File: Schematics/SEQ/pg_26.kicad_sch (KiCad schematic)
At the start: 4 parts, among them U2701 F374, U2702 F374, U2703 F374, U2704 F20

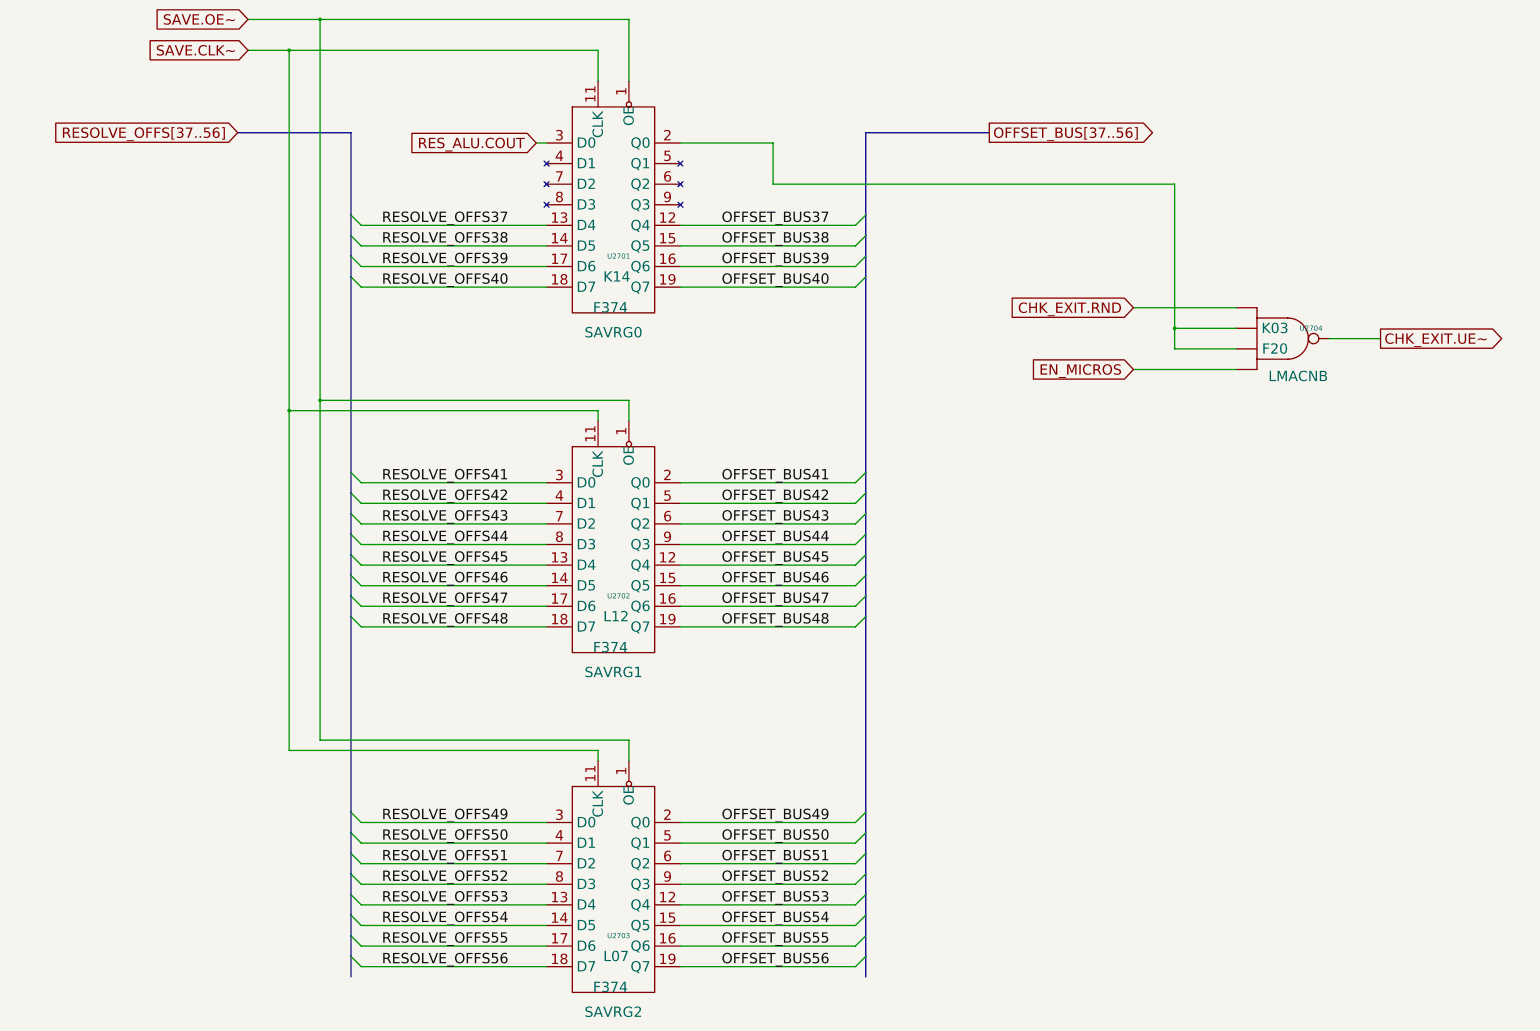
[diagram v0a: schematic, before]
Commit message: Much work on SEQ
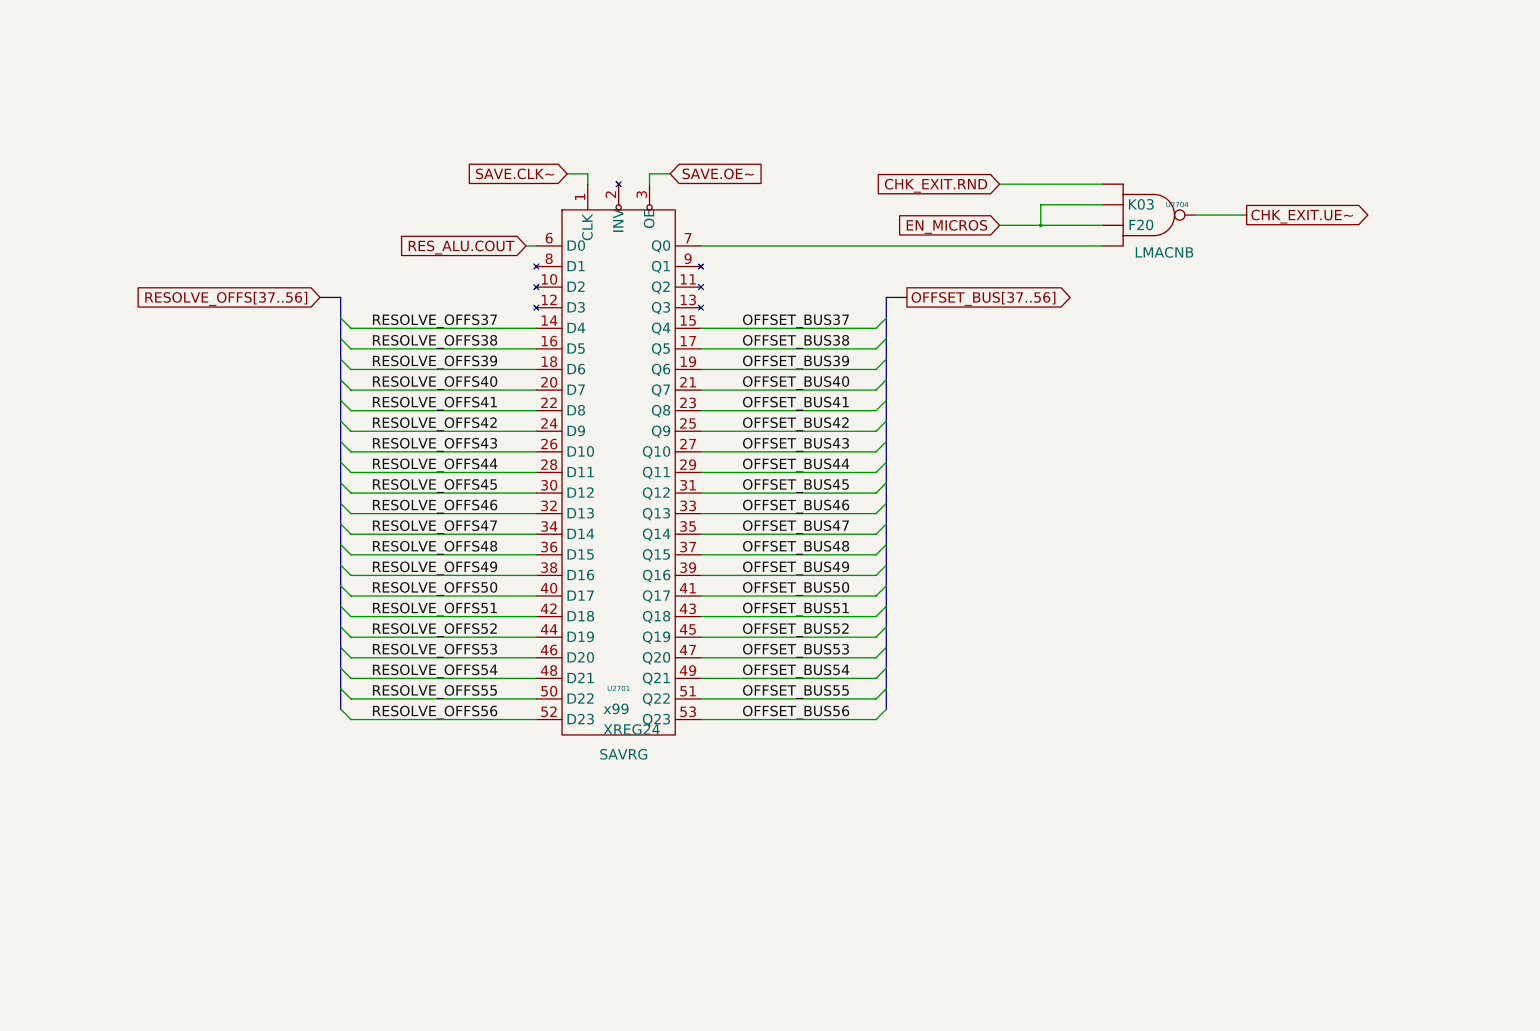
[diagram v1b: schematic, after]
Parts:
- removed U2702, U2703: F374, symbol r1000:F374
- U2701: value F374 -> XREG24; symbol r1000:F374 -> r1000:XREG24; Location K14 -> x99; Name SAVRG0 -> SAVRG
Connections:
- net EN_MICROS: now also U2704.2 (D1), U2704.4 (D2); no longer U2704.5 (D3)
- net OFFSET_BUS37: now also U2701.15 (Q4); no longer U2701.12 (Q4)
- net OFFSET_BUS38: now also U2701.17 (Q5); no longer U2701.15 (Q5)
- net OFFSET_BUS39: now also U2701.19 (Q6); no longer U2701.16 (Q6)
- net OFFSET_BUS40: now also U2701.21 (Q7); no longer U2701.19 (Q7)
- net OFFSET_BUS41: now also U2701.23 (Q8)
- net OFFSET_BUS42: now also U2701.25 (Q9)
- net OFFSET_BUS43: now also U2701.27 (Q10)
- net OFFSET_BUS44: now also U2701.29 (Q11)
- net OFFSET_BUS45: now also U2701.31 (Q12)
- net OFFSET_BUS46: now also U2701.33 (Q13)
- net OFFSET_BUS47: now also U2701.35 (Q14)
- net OFFSET_BUS48: now also U2701.37 (Q15)
- net OFFSET_BUS49: now also U2701.39 (Q16)
- net OFFSET_BUS50: now also U2701.41 (Q17)
- net OFFSET_BUS51: now also U2701.43 (Q18)
- net OFFSET_BUS52: now also U2701.45 (Q19)
- net OFFSET_BUS53: now also U2701.47 (Q20)
- net OFFSET_BUS54: now also U2701.49 (Q21)
- net OFFSET_BUS55: now also U2701.51 (Q22)
- net OFFSET_BUS56: now also U2701.53 (Q23)
- net RESOLVE_OFFS37: now also U2701.14 (D4); no longer U2701.13 (D4)
- net RESOLVE_OFFS38: now also U2701.16 (D5); no longer U2701.14 (D5)
- net RESOLVE_OFFS39: now also U2701.18 (D6); no longer U2701.17 (D6)
- net RESOLVE_OFFS40: now also U2701.20 (D7); no longer U2701.18 (D7)
- net RESOLVE_OFFS41: now also U2701.22 (D8)
- net RESOLVE_OFFS42: now also U2701.24 (D9)
- net RESOLVE_OFFS43: now also U2701.26 (D10)
- net RESOLVE_OFFS44: now also U2701.28 (D11)
- net RESOLVE_OFFS45: now also U2701.30 (D12)
- net RESOLVE_OFFS46: now also U2701.32 (D13)
- net RESOLVE_OFFS47: now also U2701.34 (D14)
- net RESOLVE_OFFS48: now also U2701.36 (D15)
- net RESOLVE_OFFS49: now also U2701.38 (D16)
- net RESOLVE_OFFS50: now also U2701.40 (D17)
- net RESOLVE_OFFS51: now also U2701.42 (D18)
- net RESOLVE_OFFS52: now also U2701.44 (D19)
- net RESOLVE_OFFS53: now also U2701.46 (D20)
- net RESOLVE_OFFS54: now also U2701.48 (D21)
- net RESOLVE_OFFS55: now also U2701.50 (D22)
- net RESOLVE_OFFS56: now also U2701.52 (D23)
- net RES_ALU.COUT: now also U2701.6 (D0); no longer U2701.3 (D0)
- net SAVE.CLK~: now also U2701.1 (CLK); no longer U2701.11 (CLK)
- net SAVE.OE~: now also U2701.3 (OE); no longer U2701.1 (OE)
- net at U2701.7 (Q0): now also U2704.5 (D3)
- now unconnected: U2701.2 (Q0)
- no-connect marks 6 -> 7
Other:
- moved on the sheet: U2704
